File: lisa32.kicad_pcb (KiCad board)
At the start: 2 copper layers, 29.1 x 58.3 mm, 69 parts, among them J1 USB4105-GF-A, J2 Conn_01x19, J3 Conn_01x19, Q1 SS8050-G, Q2 SS8050-G, SW1 BOOT, SW2 RST, U1 ESP32-WROOM-32, U2 FT2232HL, U3 LD1117S33TR_SOT223, U4 93C46, Y1 12MHz

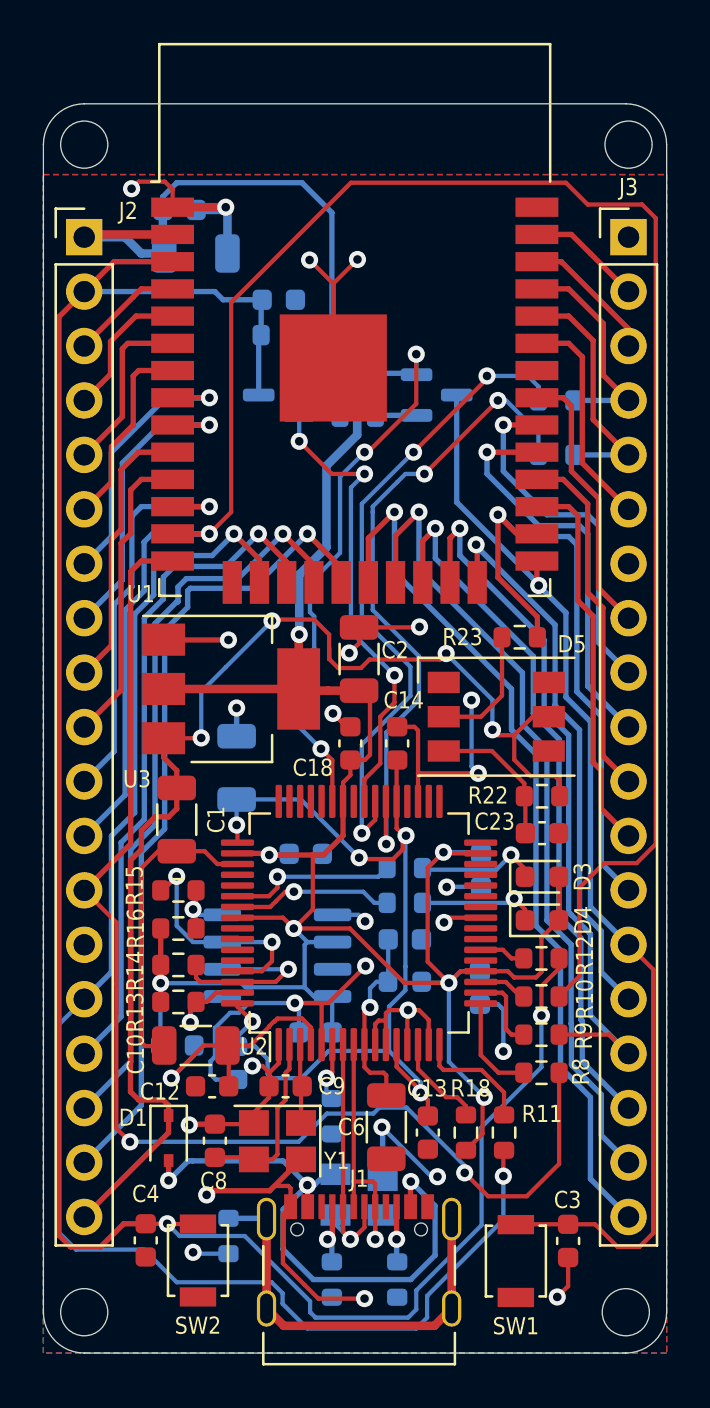
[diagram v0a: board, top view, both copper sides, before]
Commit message: v0.1.0
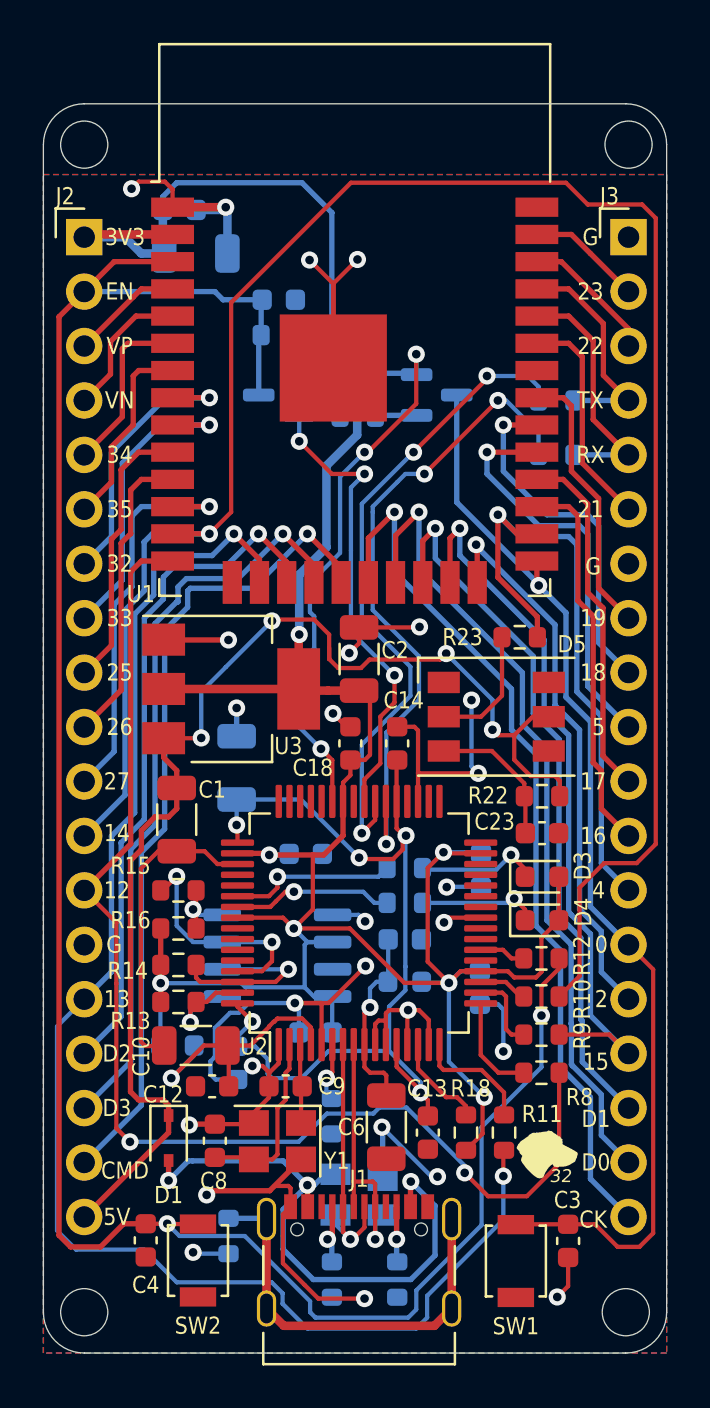
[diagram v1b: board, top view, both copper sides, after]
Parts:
- added G***: LOGO, LOGO, F.Cu at (23.5, 49.0)
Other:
- board text added: "0"
- board text added: "12"
- board text added: "13"
- board text added: "14"
- board text added: "15"
- board text added: "16"
- board text added: "17"
- board text added: "18"
- board text added: "19"
- board text added: "2"
- board text added: "21"
- board text added: "22"
- board text added: "23"
- board text added: "25"
- board text added: "26"
- board text added: "27"
- board text added: "32"
- board text added: "33"
- board text added: "34"
- board text added: "35"
- board text added: "3V3"
- board text added: "4"
- board text added: "5"
- board text added: "5V"
- board text added: "CK"
- board text added: "CMD"
- board text added: "D0"
- board text added: "D1"
- board text added: "D2"
- board text added: "D3"
- board text added: "EN"
- board text added: "G"
- board text added: "RX"
- board text added: "TX"
- board text added: "VN"
- board text added: "VP"
